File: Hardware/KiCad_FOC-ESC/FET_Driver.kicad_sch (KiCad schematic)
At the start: 1 part, among them IC1 DRV8300DPWR

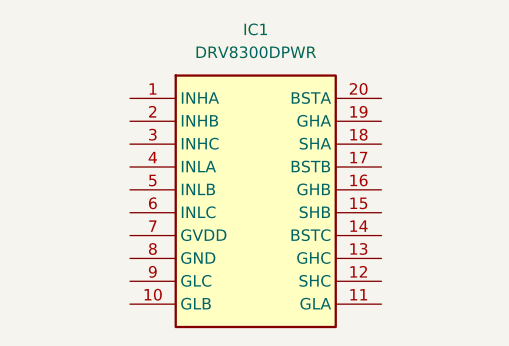
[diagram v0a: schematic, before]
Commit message: updated:schematics (#9)
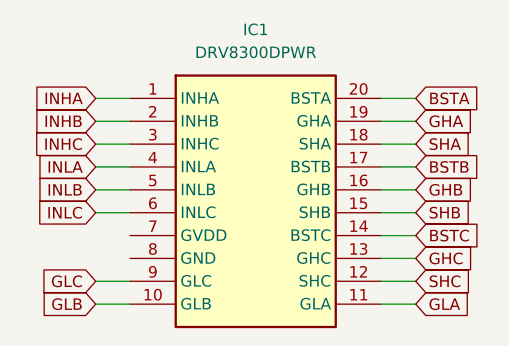
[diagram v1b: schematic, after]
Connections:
- net INHA: now reaches IC1.1 (INHA)
- net GLB: now reaches IC1.10 (GLB)
- net GLA: now reaches IC1.11 (GLA)
- net SHC: now reaches IC1.12 (SHC)
- net GHC: now reaches IC1.13 (GHC)
- net BSTC: now reaches IC1.14 (BSTC)
- net SHB: now reaches IC1.15 (SHB)
- net GHB: now reaches IC1.16 (GHB)
- net BSTB: now reaches IC1.17 (BSTB)
- net SHA: now reaches IC1.18 (SHA)
- net GHA: now reaches IC1.19 (GHA)
- net INHB: now reaches IC1.2 (INHB)
- net BSTA: now reaches IC1.20 (BSTA)
- net INHC: now reaches IC1.3 (INHC)
- net INLA: now reaches IC1.4 (INLA)
- net INLB: now reaches IC1.5 (INLB)
- net INLC: now reaches IC1.6 (INLC)
- net GLC: now reaches IC1.9 (GLC)
